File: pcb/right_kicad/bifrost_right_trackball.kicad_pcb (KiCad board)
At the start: 2 copper layers, 18.6 x 20.2 mm, 12 parts, among them J1 Conn_01x06, U1 PMW3610, U2 MCP1700x-180xxTT

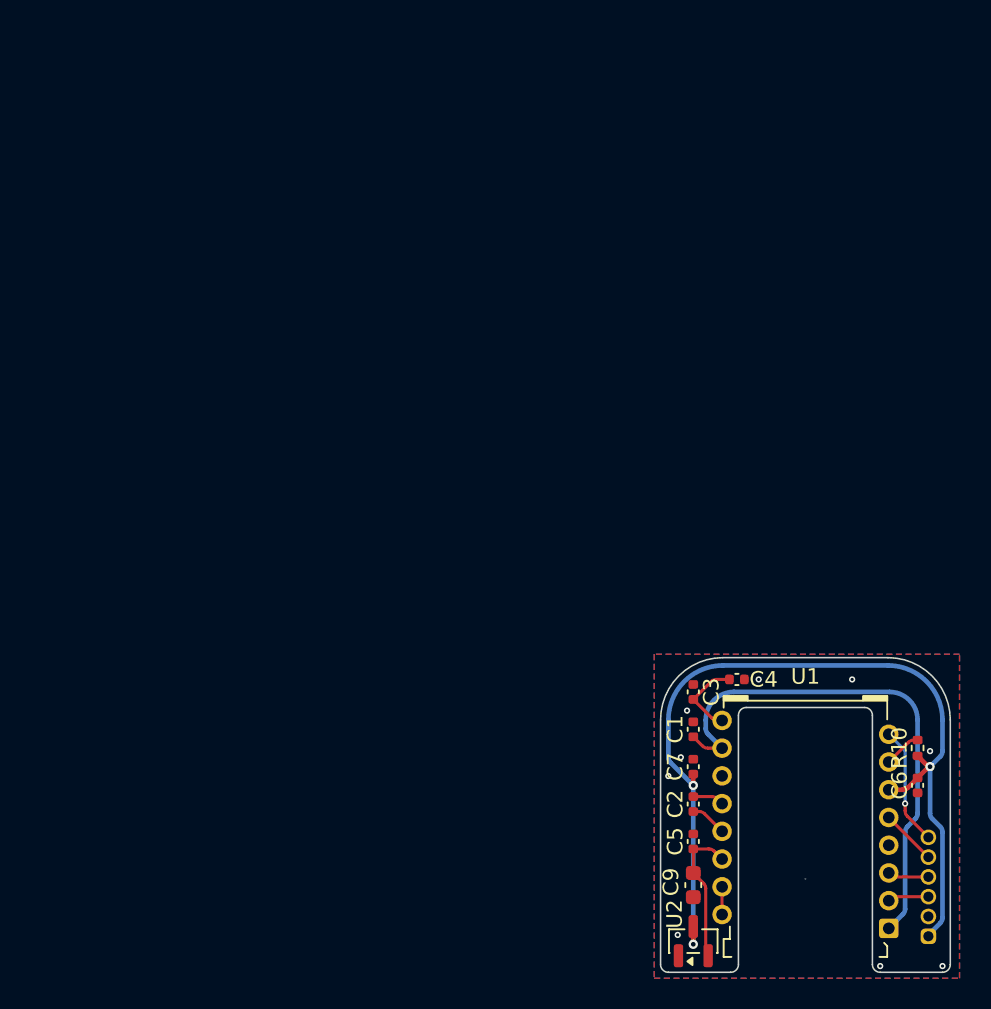
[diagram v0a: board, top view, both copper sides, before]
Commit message: Update PCB and case designs
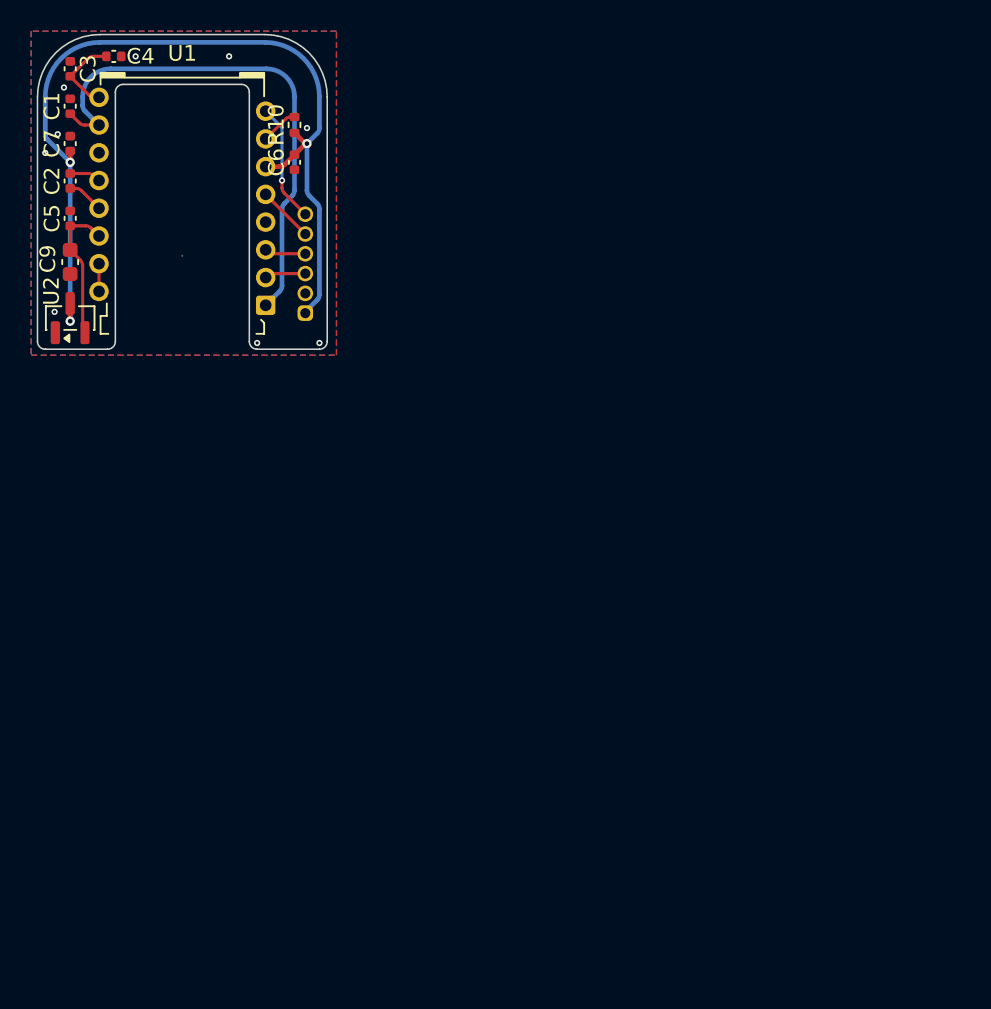
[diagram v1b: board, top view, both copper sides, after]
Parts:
- moved C1 56.6 mm to (91.7, 49.6)
- moved C2 56.6 mm to (91.7, 54.4)
- moved C3 56.6 mm to (91.7, 47.2)
- moved C7 56.6 mm to (91.7, 52.0)
- moved C9 56.6 mm to (91.7, 59.6)
- moved J1 56.6 mm to (106.8, 62.9)
- moved U2 56.6 mm to (91.7, 63.2)
- moved C5 56.6 mm to (91.7, 56.8)
- moved C4 56.6 mm to (94.5, 46.4)
- moved U1 56.6 mm to (98.9, 59.2)
- moved C6 56.6 mm to (106.1, 53.2)
- moved R10 56.6 mm to (106.1, 50.8)
